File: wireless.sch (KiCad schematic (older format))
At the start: 22 parts, among them U6 NRF24L01+, X2 16MHz 10ppm

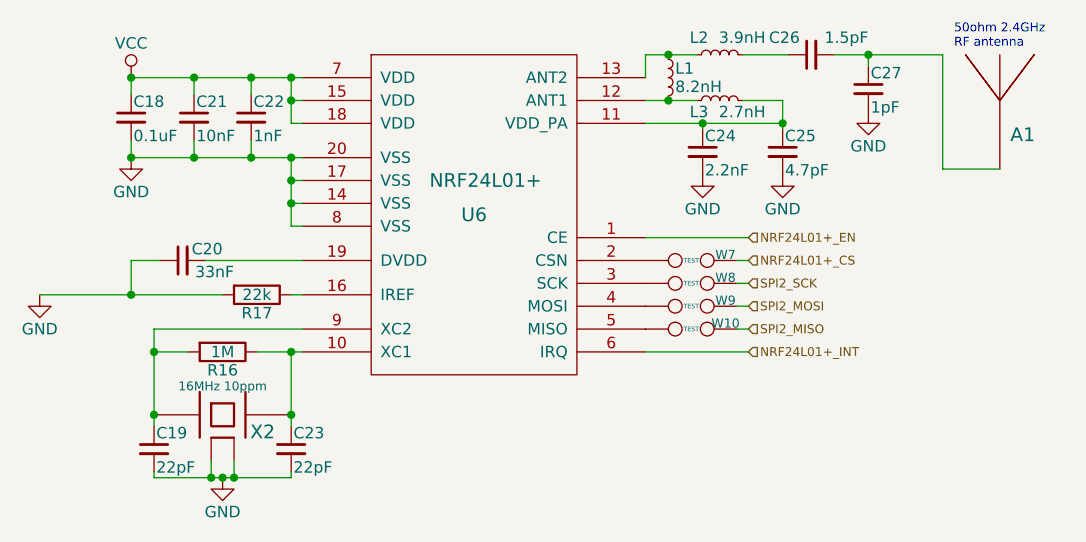
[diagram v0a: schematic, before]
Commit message: Revert "Remove SD card"
This reverts commit 4a1918bee256f93cb8d66746410e6c192988175c.
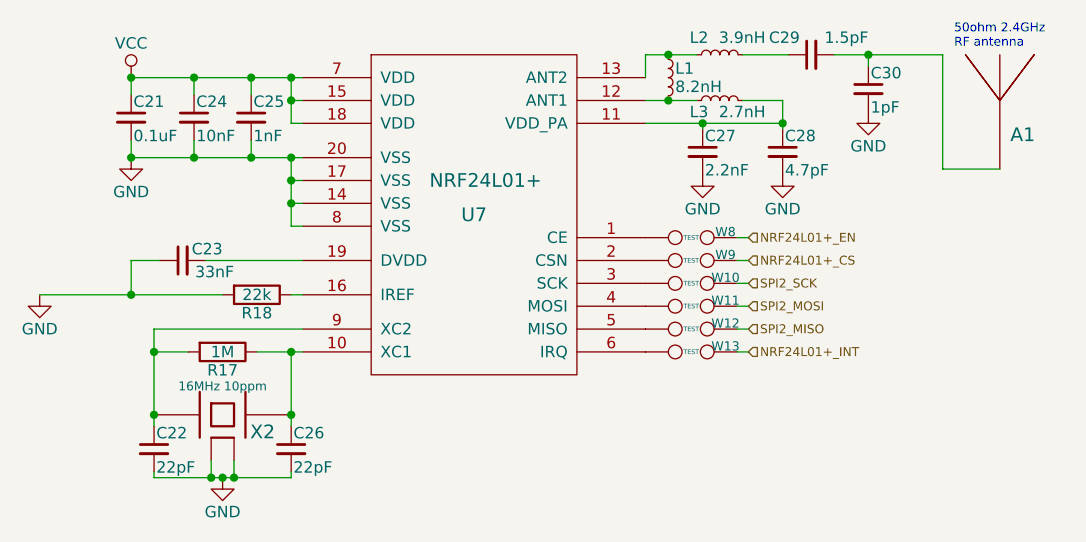
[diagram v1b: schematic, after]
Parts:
- added W13, W8: TEST, _std:Measurement_Point_Round-SMD-Pad_Small, symbol TEST
- renumbered C18 to C21, C19 to C22, C20 to C23, C21 to C24, C22 to C25, C23 to C26, C24 to C27, C25 to C28, C26 to C29, C27 to C30, R16 to R17, R17 to R18, U6 to U7, W8 to W10, W9 to W11, W10 to W12, W7 to W9
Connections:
- net NRF24L01+_EN: now also W8.2; no longer U7.1 (CE)
- net NRF24L01+_INT: now also W13.2; no longer U7.6 (IRQ)
- new net: U7.1 (CE), W8.1
- new net: U7.6 (IRQ), W13.1
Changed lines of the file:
@@
 $EndDescr
 $Comp
-L NRF24R01+ U6
+L NRF24R01+ U7
 U 1 1 55438B0D
 P 5175 3125
-F 0 "U6" H 5175 3125 60  0000 C CNN
+F 0 "U7" H 5175 3125 60  0000 C CNN
 F 1 "NRF24L01+" H 5225 3275 60  0000 C CNN
 F 2 "Housings_DFN_QFN:QFN-20-1EP_4x4mm_Pitch0.5mm" H 5175 3125 60  0001 C CNN
@@
 $EndComp
 $Comp
-L VCC #PWR032
+L VCC #PWR041
 U 1 1 55438B1A
 P 3675 2525
-F 0 "#PWR032" H 3675 2375 50  0001 C CNN
+F 0 "#PWR041" H 3675 2375 50  0001 C CNN
 F 1 "VCC" H 3675 2675 50  0000 C CNN
 F 2 "" H 3675 2525 60  0000 C CNN
@@
 $EndComp
 $Comp
-L GND #PWR033
+L GND #PWR042
 U 1 1 55438B20
 P 3275 3475
-F 0 "#PWR033" H 3275 3225 50  0001 C CNN
+F 0 "#PWR042" H 3275 3225 50  0001 C CNN
 F 1 "GND" H 3275 3325 50  0000 C CNN
 F 2 "" H 3275 3475 60  0000 C CNN
@@
 $EndComp
 $Comp
-L R R17
+L R R18
 U 1 1 55438B26
 P 4225 3475
-F 0 "R17" V 4305 3475 50  0000 C CNN
+F 0 "R18" V 4305 3475 50  0000 C CNN
 F 1 "22k" V 4225 3475 50  0000 C CNN
 F 2 "_std:_0402" V 4155 3475 30  0001 C CNN
@@
 $EndComp
 $Comp
-L GND #PWR034
+L GND #PWR043
 U 1 1 55438B2D
 P 4075 4275
-F 0 "#PWR034" H 4075 4025 50  0001 C CNN
+F 0 "#PWR043" H 4075 4025 50  0001 C CNN
 F 1 "GND" H 4075 4125 50  0000 C CNN
 F 2 "" H 4075 4275 60  0000 C CNN
@@
 $EndComp
 $Comp
-L GND #PWR035
+L GND #PWR044
 U 1 1 55438B33
 P 6175 2950
-F 0 "#PWR035" H 6175 2700 50  0001 C CNN
+F 0 "#PWR044" H 6175 2700 50  0001 C CNN
 F 1 "GND" H 6175 2800 50  0000 C CNN
 F 2 "" H 6175 2950 60  0000 C CNN
@@
 $EndComp
 $Comp
-L GND #PWR036
+L GND #PWR045
 U 1 1 55438B39
 P 6525 2950
-F 0 "#PWR036" H 6525 2700 50  0001 C CNN
+F 0 "#PWR045" H 6525 2700 50  0001 C CNN
 F 1 "GND" H 6525 2800 50  0000 C CNN
 F 2 "" H 6525 2950 60  0000 C CNN
@@
 $EndComp
 $Comp
-L C_Small C26
+L C_Small C29
 U 1 1 55438B54
 P 6650 2425
-F 0 "C26" V 6725 2475 50  0000 L CNN
+F 0 "C29" V 6725 2475 50  0000 L CNN
 F 1 "1.5pF" V 6725 2175 50  0000 L CNN
 F 2 "_std:_0402" H 6650 2425 60  0001 C CNN
@@
 $EndComp
 $Comp
-L GND #PWR037
+L GND #PWR046
 U 1 1 55438B5B
 P 6900 2675
-F 0 "#PWR037" H 6900 2425 50  0001 C CNN
+F 0 "#PWR046" H 6900 2425 50  0001 C CNN
 F 1 "GND" H 6900 2525 50  0000 C CNN
 F 2 "" H 6900 2675 60  0000 C CNN
@@
 $EndComp
 $Comp
-L C_Small C24
+L C_Small C27
 U 1 1 55438B61
 P 6175 2850
-F 0 "C24" H 6185 2920 50  0000 L CNN
+F 0 "C27" H 6185 2920 50  0000 L CNN
 F 1 "2.2nF" H 6185 2770 50  0000 L CNN
 F 2 "_std:_0402" H 6175 2850 60  0001 C CNN
@@
 $EndComp
 $Comp
-L C_Small C25
+L C_Small C28
 U 1 1 55438B68
 P 6525 2850
-F 0 "C25" H 6535 2920 50  0000 L CNN
+F 0 "C28" H 6535 2920 50  0000 L CNN
 F 1 "4.7pF" H 6535 2770 50  0000 L CNN
 F 2 "_std:_0402" H 6525 2850 60  0001 C CNN
@@
 $EndComp
 $Comp
-L R R16
+L R R17
 U 1 1 55438B76
 P 4075 3725
-F 0 "R16" V 4155 3725 50  0000 C CNN
+F 0 "R17" V 4155 3725 50  0000 C CNN
 F 1 "1M" V 4075 3725 50  0000 C CNN
 F 2 "_std:_0402" V 4005 3725 30  0001 C CNN
@@
 $EndComp
 $Comp
-L C_Small C19
+L C_Small C22
 U 1 1 55438B7D
 P 3775 4150
-F 0 "C19" H 3785 4220 50  0000 L CNN
+F 0 "C22" H 3785 4220 50  0000 L CNN
 F 1 "22pF" H 3785 4070 50  0000 L CNN
 F 2 "_std:_0402" H 3775 4150 60  0001 C CNN
@@
 $EndComp
 $Comp
-L C_Small C23
+L C_Small C26
 U 1 1 55438B84
 P 4375 4150
-F 0 "C23" H 4385 4220 50  0000 L CNN
+F 0 "C26" H 4385 4220 50  0000 L CNN
 F 1 "22pF" H 4385 4070 50  0000 L CNN
 F 2 "_std:_0402" H 4375 4150 60  0001 C CNN
@@
 $EndComp
 $Comp
-L C_Small C20
+L C_Small C23
 U 1 1 55438B8B
 P 3900 3325
-F 0 "C20" V 3950 3150 50  0000 L CNN
+F 0 "C23" V 3950 3150 50  0000 L CNN
 F 1 "33nF" V 3850 3100 50  0000 L CNN
 F 2 "_std:_0402" H 3900 3325 60  0001 C CNN
@@
 $EndComp
 $Comp
-L C_Small C27
+L C_Small C30
 U 1 1 55438B92
 P 6900 2575
-F 0 "C27" H 6910 2645 50  0000 L CNN
+F 0 "C30" H 6910 2645 50  0000 L CNN
 F 1 "1pF" H 6910 2495 50  0000 L CNN
 F 2 "_std:_0402" H 6900 2575 60  0001 C CNN
@@
 $EndComp
 $Comp
-L C_Small C18
+L C_Small C21
 U 1 1 55438B99
 P 3675 2700
-F 0 "C18" H 3685 2770 50  0000 L CNN
+F 0 "C21" H 3685 2770 50  0000 L CNN
 F 1 "0.1uF" H 3685 2620 50  0000 L CNN
 F 2 "_std:_0402" H 3675 2700 60  0001 C CNN
@@
 $EndComp
 $Comp
-L C_Small C22
+L C_Small C25
 U 1 1 55438BA0
 P 4200 2700
-F 0 "C22" H 4210 2770 50  0000 L CNN
+F 0 "C25" H 4210 2770 50  0000 L CNN
 F 1 "1nF" H 4210 2620 50  0000 L CNN
 F 2 "_std:_0402" H 4200 2700 60  0001 C CNN
@@
 $EndComp
 $Comp
-L GND #PWR038
+L GND #PWR047
 U 1 1 55438BA7
 P 3675 2875
-F 0 "#PWR038" H 3675 2625 50  0001 C CNN
+F 0 "#PWR047" H 3675 2625 50  0001 C CNN
 F 1 "GND" H 3675 2725 50  0000 C CNN
 F 2 "" H 3675 2875 60  0000 C CNN
@@
 	4225 3725 4425 3725
 Wire Wire Line
-	6375 3725 5925 3725
-Wire Wire Line
-	6375 3225 5925 3225
+	6375 3725 6325 3725
+Wire Wire Line
+	6375 3225 6325 3225
 Wire Wire Line
 	6325 3625 6375 3625
@@
 Connection ~ 4200 2875
 $Comp
-L C_Small C21
+L C_Small C24
 U 1 1 55438BFC
 P 3950 2700
-F 0 "C21" H 3960 2770 50  0000 L CNN
+F 0 "C24" H 3960 2770 50  0000 L CNN
 F 1 "10nF" H 3960 2620 50  0000 L CNN
 F 2 "_std:_0402" H 3950 2700 60  0001 C CNN
@@
 NRF24L01+_INT
 $Comp
-L TEST W7
+L TEST W8
+U 1 1 5579456F
+P 6125 3225
+F 0 "W8" H 6275 3250 40  0000 C CNN
+F 1 "TEST" H 6125 3225 20  0000 C CNN
+F 2 "_std:Measurement_Point_Round-SMD-Pad_Small" H 6125 3225 60  0001 C CNN
+F 3 "" H 6125 3225 60  0000 C CNN
+	1    6125 3225
+	1    0    0    -1
+$EndComp
+$Comp
+L TEST W9
 U 1 1 5579499D
 P 6125 3325
-F 0 "W7" H 6275 3350 40  0000 C CNN
+F 0 "W9" H 6275 3350 40  0000 C CNN
 F 1 "TEST" H 6125 3325 20  0000 C CNN
 F 2 "_std:Measurement_Point_Round-SMD-Pad_Small" H 6125 3325 60  0001 C CNN
@@
 $EndComp
 $Comp
-L TEST W8
+L TEST W10
 U 1 1 557949DF
 P 6125 3425
-F 0 "W8" H 6275 3450 40  0000 C CNN
+F 0 "W10" H 6275 3450 40  0000 C CNN
 F 1 "TEST" H 6125 3425 20  0000 C CNN
 F 2 "_std:Measurement_Point_Round-SMD-Pad_Small" H 6125 3425 60  0001 C CNN
@@
 $EndComp
 $Comp
-L TEST W9
+L TEST W11
 U 1 1 55794A1F
 P 6125 3525
-F 0 "W9" H 6275 3550 40  0000 C CNN
+F 0 "W11" H 6275 3550 40  0000 C CNN
 F 1 "TEST" H 6125 3525 20  0000 C CNN
 F 2 "_std:Measurement_Point_Round-SMD-Pad_Small" H 6125 3525 60  0001 C CNN
@@
 $EndComp
 $Comp
-L TEST W10
+L TEST W12
 U 1 1 55794A65
 P 6125 3625
-F 0 "W10" H 6275 3650 40  0000 C CNN
+F 0 "W12" H 6275 3650 40  0000 C CNN
 F 1 "TEST" H 6125 3625 20  0000 C CNN
 F 2 "_std:Measurement_Point_Round-SMD-Pad_Small" H 6125 3625 60  0001 C CNN
@@
 	1    0    0    -1
 $EndComp
+$Comp
+L TEST W13
+U 1 1 55794AA9
+P 6125 3725
+F 0 "W13" H 6275 3750 40  0000 C CNN
+F 1 "TEST" H 6125 3725 20  0000 C CNN
+F 2 "_std:Measurement_Point_Round-SMD-Pad_Small" H 6125 3725 60  0001 C CNN
+F 3 "" H 6125 3725 60  0000 C CNN
+	1    6125 3725
+	1    0    0    -1
+$EndComp

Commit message: Remove SD card
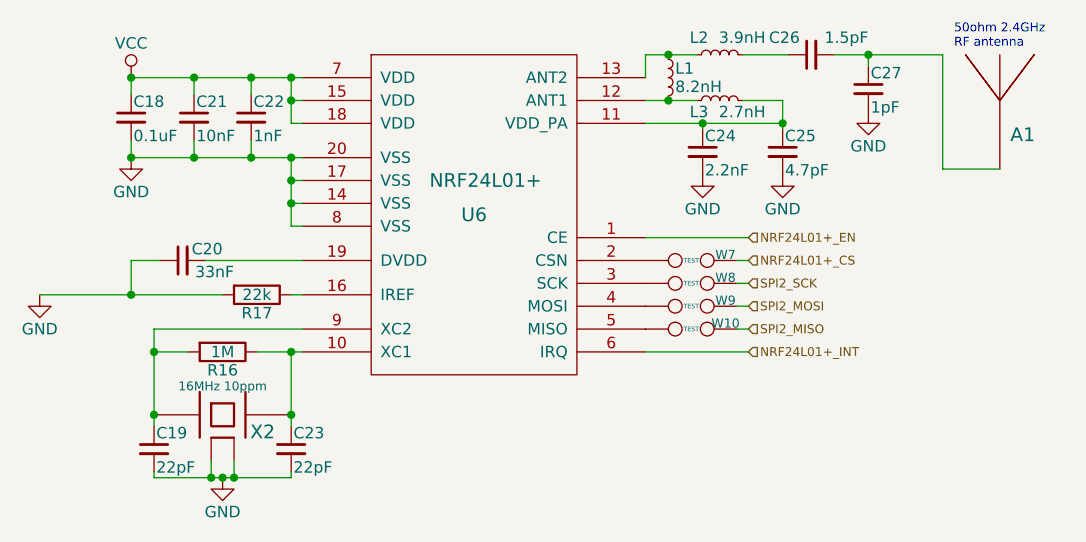
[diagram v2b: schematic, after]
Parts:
- removed W13, W8: TEST, _std:Measurement_Point_Round-SMD-Pad_Small, symbol TEST
- renumbered C21 to C18, C22 to C19, C23 to C20, C24 to C21, C25 to C22, C26 to C23, C27 to C24, C28 to C25, C29 to C26, C30 to C27, R17 to R16, R18 to R17, U7 to U6, W12 to W10, W9 to W7, W10 to W8, W11 to W9
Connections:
- net NRF24L01+_EN: now also U6.1 (CE)
- net NRF24L01+_INT: now also U6.6 (IRQ)
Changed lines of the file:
@@
 $EndDescr
 $Comp
-L NRF24R01+ U7
+L NRF24R01+ U6
 U 1 1 55438B0D
 P 5175 3125
-F 0 "U7" H 5175 3125 60  0000 C CNN
+F 0 "U6" H 5175 3125 60  0000 C CNN
 F 1 "NRF24L01+" H 5225 3275 60  0000 C CNN
 F 2 "Housings_DFN_QFN:QFN-20-1EP_4x4mm_Pitch0.5mm" H 5175 3125 60  0001 C CNN
@@
 $EndComp
 $Comp
-L VCC #PWR041
+L VCC #PWR032
 U 1 1 55438B1A
 P 3675 2525
-F 0 "#PWR041" H 3675 2375 50  0001 C CNN
+F 0 "#PWR032" H 3675 2375 50  0001 C CNN
 F 1 "VCC" H 3675 2675 50  0000 C CNN
 F 2 "" H 3675 2525 60  0000 C CNN
@@
 $EndComp
 $Comp
-L GND #PWR042
+L GND #PWR033
 U 1 1 55438B20
 P 3275 3475
-F 0 "#PWR042" H 3275 3225 50  0001 C CNN
+F 0 "#PWR033" H 3275 3225 50  0001 C CNN
 F 1 "GND" H 3275 3325 50  0000 C CNN
 F 2 "" H 3275 3475 60  0000 C CNN
@@
 $EndComp
 $Comp
-L R R18
+L R R17
 U 1 1 55438B26
 P 4225 3475
-F 0 "R18" V 4305 3475 50  0000 C CNN
+F 0 "R17" V 4305 3475 50  0000 C CNN
 F 1 "22k" V 4225 3475 50  0000 C CNN
 F 2 "_std:_0402" V 4155 3475 30  0001 C CNN
@@
 $EndComp
 $Comp
-L GND #PWR043
+L GND #PWR034
 U 1 1 55438B2D
 P 4075 4275
-F 0 "#PWR043" H 4075 4025 50  0001 C CNN
+F 0 "#PWR034" H 4075 4025 50  0001 C CNN
 F 1 "GND" H 4075 4125 50  0000 C CNN
 F 2 "" H 4075 4275 60  0000 C CNN
@@
 $EndComp
 $Comp
-L GND #PWR044
+L GND #PWR035
 U 1 1 55438B33
 P 6175 2950
-F 0 "#PWR044" H 6175 2700 50  0001 C CNN
+F 0 "#PWR035" H 6175 2700 50  0001 C CNN
 F 1 "GND" H 6175 2800 50  0000 C CNN
 F 2 "" H 6175 2950 60  0000 C CNN
@@
 $EndComp
 $Comp
-L GND #PWR045
+L GND #PWR036
 U 1 1 55438B39
 P 6525 2950
-F 0 "#PWR045" H 6525 2700 50  0001 C CNN
+F 0 "#PWR036" H 6525 2700 50  0001 C CNN
 F 1 "GND" H 6525 2800 50  0000 C CNN
 F 2 "" H 6525 2950 60  0000 C CNN
@@
 $EndComp
 $Comp
-L C_Small C29
+L C_Small C26
 U 1 1 55438B54
 P 6650 2425
-F 0 "C29" V 6725 2475 50  0000 L CNN
+F 0 "C26" V 6725 2475 50  0000 L CNN
 F 1 "1.5pF" V 6725 2175 50  0000 L CNN
 F 2 "_std:_0402" H 6650 2425 60  0001 C CNN
@@
 $EndComp
 $Comp
-L GND #PWR046
+L GND #PWR037
 U 1 1 55438B5B
 P 6900 2675
-F 0 "#PWR046" H 6900 2425 50  0001 C CNN
+F 0 "#PWR037" H 6900 2425 50  0001 C CNN
 F 1 "GND" H 6900 2525 50  0000 C CNN
 F 2 "" H 6900 2675 60  0000 C CNN
@@
 $EndComp
 $Comp
-L C_Small C27
+L C_Small C24
 U 1 1 55438B61
 P 6175 2850
-F 0 "C27" H 6185 2920 50  0000 L CNN
+F 0 "C24" H 6185 2920 50  0000 L CNN
 F 1 "2.2nF" H 6185 2770 50  0000 L CNN
 F 2 "_std:_0402" H 6175 2850 60  0001 C CNN
@@
 $EndComp
 $Comp
-L C_Small C28
+L C_Small C25
 U 1 1 55438B68
 P 6525 2850
-F 0 "C28" H 6535 2920 50  0000 L CNN
+F 0 "C25" H 6535 2920 50  0000 L CNN
 F 1 "4.7pF" H 6535 2770 50  0000 L CNN
 F 2 "_std:_0402" H 6525 2850 60  0001 C CNN
@@
 $EndComp
 $Comp
-L R R17
+L R R16
 U 1 1 55438B76
 P 4075 3725
-F 0 "R17" V 4155 3725 50  0000 C CNN
+F 0 "R16" V 4155 3725 50  0000 C CNN
 F 1 "1M" V 4075 3725 50  0000 C CNN
 F 2 "_std:_0402" V 4005 3725 30  0001 C CNN
@@
 $EndComp
 $Comp
-L C_Small C22
+L C_Small C19
 U 1 1 55438B7D
 P 3775 4150
-F 0 "C22" H 3785 4220 50  0000 L CNN
+F 0 "C19" H 3785 4220 50  0000 L CNN
 F 1 "22pF" H 3785 4070 50  0000 L CNN
 F 2 "_std:_0402" H 3775 4150 60  0001 C CNN
@@
 $EndComp
 $Comp
-L C_Small C26
+L C_Small C23
 U 1 1 55438B84
 P 4375 4150
-F 0 "C26" H 4385 4220 50  0000 L CNN
+F 0 "C23" H 4385 4220 50  0000 L CNN
 F 1 "22pF" H 4385 4070 50  0000 L CNN
 F 2 "_std:_0402" H 4375 4150 60  0001 C CNN
@@
 $EndComp
 $Comp
-L C_Small C23
+L C_Small C20
 U 1 1 55438B8B
 P 3900 3325
-F 0 "C23" V 3950 3150 50  0000 L CNN
+F 0 "C20" V 3950 3150 50  0000 L CNN
 F 1 "33nF" V 3850 3100 50  0000 L CNN
 F 2 "_std:_0402" H 3900 3325 60  0001 C CNN
@@
 $EndComp
 $Comp
-L C_Small C30
+L C_Small C27
 U 1 1 55438B92
 P 6900 2575
-F 0 "C30" H 6910 2645 50  0000 L CNN
+F 0 "C27" H 6910 2645 50  0000 L CNN
 F 1 "1pF" H 6910 2495 50  0000 L CNN
 F 2 "_std:_0402" H 6900 2575 60  0001 C CNN
@@
 $EndComp
 $Comp
-L C_Small C21
+L C_Small C18
 U 1 1 55438B99
 P 3675 2700
-F 0 "C21" H 3685 2770 50  0000 L CNN
+F 0 "C18" H 3685 2770 50  0000 L CNN
 F 1 "0.1uF" H 3685 2620 50  0000 L CNN
 F 2 "_std:_0402" H 3675 2700 60  0001 C CNN
@@
 $EndComp
 $Comp
-L C_Small C25
+L C_Small C22
 U 1 1 55438BA0
 P 4200 2700
-F 0 "C25" H 4210 2770 50  0000 L CNN
+F 0 "C22" H 4210 2770 50  0000 L CNN
 F 1 "1nF" H 4210 2620 50  0000 L CNN
 F 2 "_std:_0402" H 4200 2700 60  0001 C CNN
@@
 $EndComp
 $Comp
-L GND #PWR047
+L GND #PWR038
 U 1 1 55438BA7
 P 3675 2875
-F 0 "#PWR047" H 3675 2625 50  0001 C CNN
+F 0 "#PWR038" H 3675 2625 50  0001 C CNN
 F 1 "GND" H 3675 2725 50  0000 C CNN
 F 2 "" H 3675 2875 60  0000 C CNN
@@
 	4225 3725 4425 3725
 Wire Wire Line
-	6375 3725 6325 3725
-Wire Wire Line
-	6375 3225 6325 3225
+	6375 3725 5925 3725
+Wire Wire Line
+	6375 3225 5925 3225
 Wire Wire Line
 	6325 3625 6375 3625
@@
 Connection ~ 4200 2875
 $Comp
-L C_Small C24
+L C_Small C21
 U 1 1 55438BFC
 P 3950 2700
-F 0 "C24" H 3960 2770 50  0000 L CNN
+F 0 "C21" H 3960 2770 50  0000 L CNN
 F 1 "10nF" H 3960 2620 50  0000 L CNN
 F 2 "_std:_0402" H 3950 2700 60  0001 C CNN
@@
 NRF24L01+_INT
 $Comp
-L TEST W8
-U 1 1 5579456F
-P 6125 3225
-F 0 "W8" H 6275 3250 40  0000 C CNN
-F 1 "TEST" H 6125 3225 20  0000 C CNN
-F 2 "_std:Measurement_Point_Round-SMD-Pad_Small" H 6125 3225 60  0001 C CNN
-F 3 "" H 6125 3225 60  0000 C CNN
-	1    6125 3225
-	1    0    0    -1
-$EndComp
-$Comp
-L TEST W9
+L TEST W7
 U 1 1 5579499D
 P 6125 3325
-F 0 "W9" H 6275 3350 40  0000 C CNN
+F 0 "W7" H 6275 3350 40  0000 C CNN
 F 1 "TEST" H 6125 3325 20  0000 C CNN
 F 2 "_std:Measurement_Point_Round-SMD-Pad_Small" H 6125 3325 60  0001 C CNN
@@
 $EndComp
 $Comp
-L TEST W10
+L TEST W8
 U 1 1 557949DF
 P 6125 3425
-F 0 "W10" H 6275 3450 40  0000 C CNN
+F 0 "W8" H 6275 3450 40  0000 C CNN
 F 1 "TEST" H 6125 3425 20  0000 C CNN
 F 2 "_std:Measurement_Point_Round-SMD-Pad_Small" H 6125 3425 60  0001 C CNN
@@
 $EndComp
 $Comp
-L TEST W11
+L TEST W9
 U 1 1 55794A1F
 P 6125 3525
-F 0 "W11" H 6275 3550 40  0000 C CNN
+F 0 "W9" H 6275 3550 40  0000 C CNN
 F 1 "TEST" H 6125 3525 20  0000 C CNN
 F 2 "_std:Measurement_Point_Round-SMD-Pad_Small" H 6125 3525 60  0001 C CNN
@@
 $EndComp
 $Comp
-L TEST W12
+L TEST W10
 U 1 1 55794A65
 P 6125 3625
-F 0 "W12" H 6275 3650 40  0000 C CNN
+F 0 "W10" H 6275 3650 40  0000 C CNN
 F 1 "TEST" H 6125 3625 20  0000 C CNN
 F 2 "_std:Measurement_Point_Round-SMD-Pad_Small" H 6125 3625 60  0001 C CNN
@@
 	1    0    0    -1
 $EndComp
-$Comp
-L TEST W13
-U 1 1 55794AA9
-P 6125 3725
-F 0 "W13" H 6275 3750 40  0000 C CNN
-F 1 "TEST" H 6125 3725 20  0000 C CNN
-F 2 "_std:Measurement_Point_Round-SMD-Pad_Small" H 6125 3725 60  0001 C CNN
-F 3 "" H 6125 3725 60  0000 C CNN
-	1    6125 3725
-	1    0    0    -1
-$EndComp
